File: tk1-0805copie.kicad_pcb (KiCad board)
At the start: 2 copper layers, 63 x 38.4 mm, 65 parts, among them P1 USB_C_Plug, U1 MCP1824T-2502EOT, U2 NCV8164ASN120T1G, U3 CH552E, U5 USBLC6-2SC6, U6 ICE40UP5K-SG48ITR, U8 W25Q80DVSNIG, U9 NCP752BSN33T1G

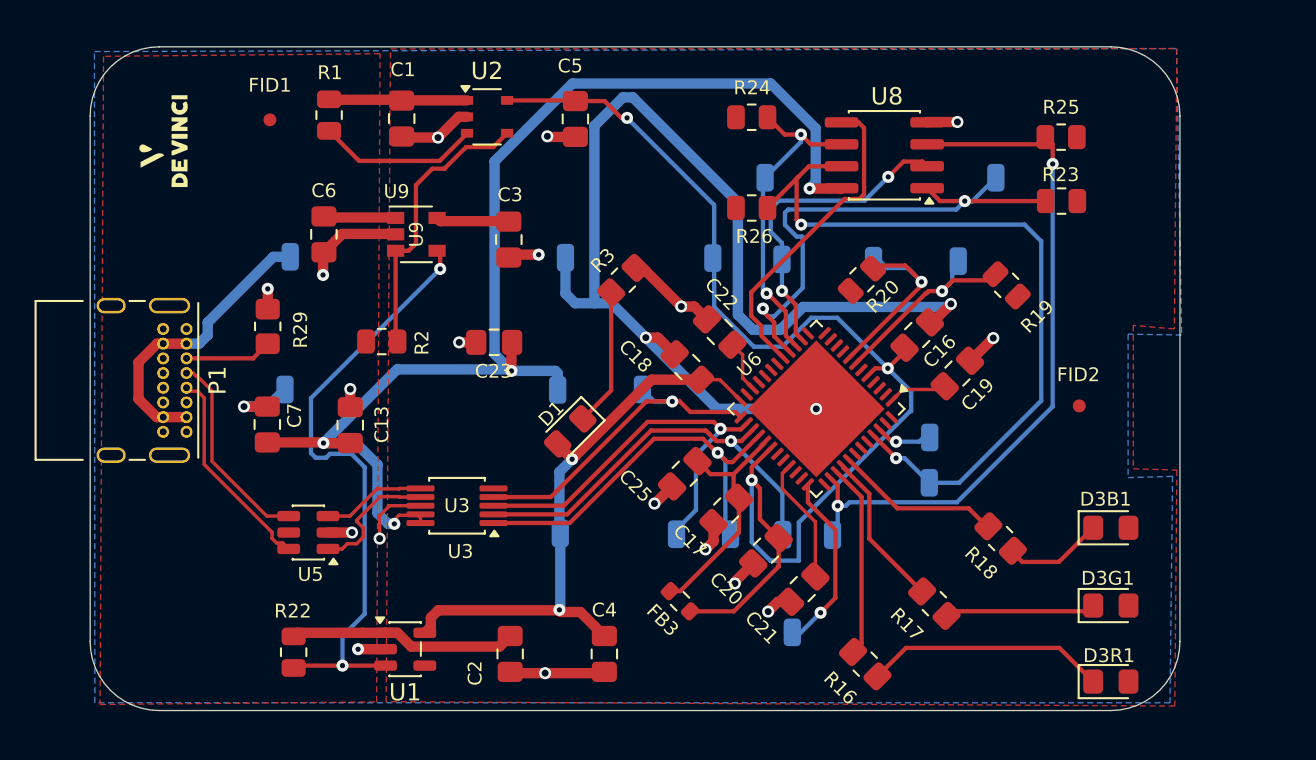
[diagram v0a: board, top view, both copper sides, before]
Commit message: Mise à jour du projet
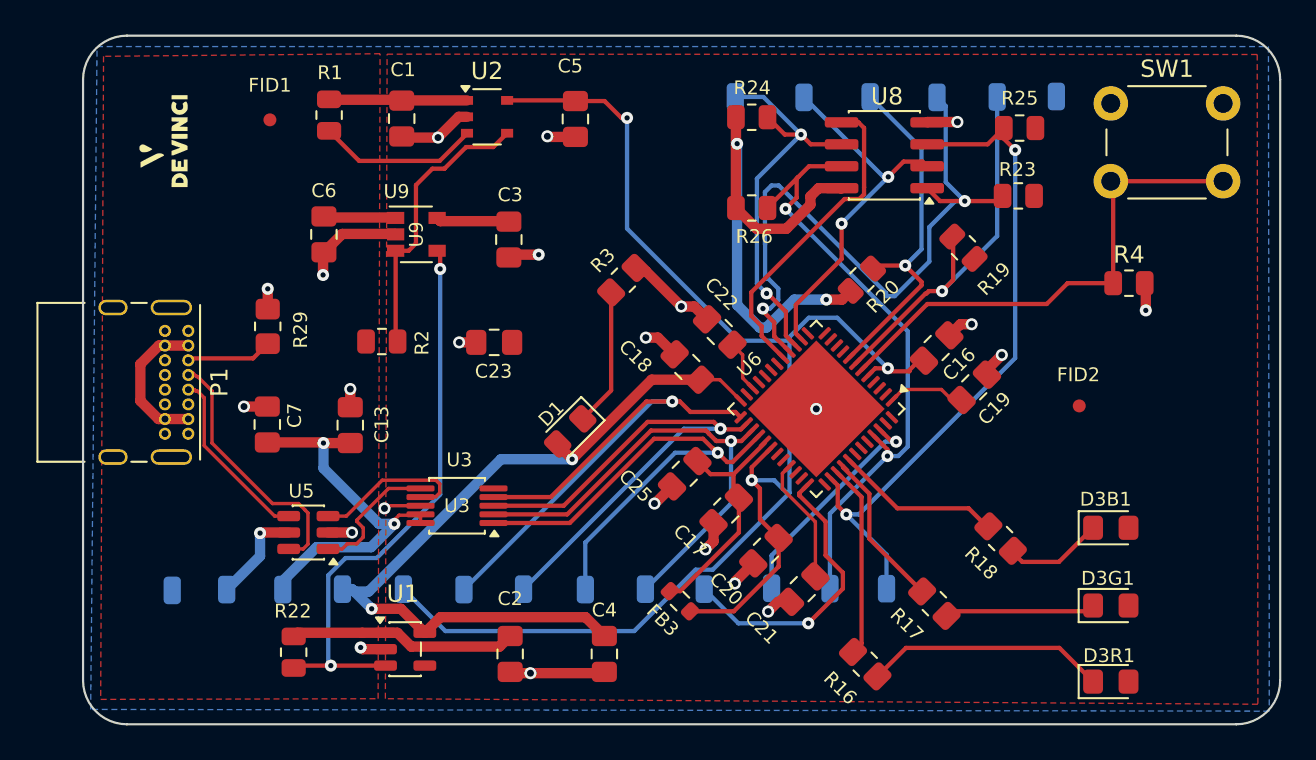
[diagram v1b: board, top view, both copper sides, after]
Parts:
- added R4: 10k, Resistor_SMD:R_0805_2012Metric, F.Cu at (138.1, 86.8)
- added SW1: SW_Push, Button_Switch_THT:SW_PUSH_6mm, F.Cu at (137.0, 76.3)
- U8: value W25Q80DVSNIG -> SST26VF080A-104I/SN
- moved TP5 29.9 mm to (133.8, 76.0)
- moved TP4 26.2 mm to (96.1, 104.5)
- moved TP2 19.7 mm to (89.1, 104.5)
- moved TP1 19.6 mm to (85.8, 104.5)
- moved TP6 15.5 mm to (99.6, 104.5)
- moved TP28 13.3 mm to (82.7, 104.5)
- moved TP3 13.0 mm to (92.5, 104.5)
- moved TP21 12.6 mm to (117.4, 104.4)
- moved TP17 9.76 mm to (130.4, 76.0)
- moved TP16 9.48 mm to (123.1, 76.0)
- moved TP15 9.46 mm to (119.2, 76.0)
- moved TP7 9.40 mm to (103.0, 104.5)
- moved TP8 8.99 mm to (106.6, 104.5)
- moved TP9 8.55 mm to (110.1, 104.5)
- moved TP20 8.40 mm to (120.8, 104.4)
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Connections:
- U3 pad 6: INT_USB_D- -> INT_USB_D+
- U3 pad 7: INT_USB_D+ -> INT_USB_D-
- U5 pad 4: /USB to Serial converter/INT_USB_IN_D+ -> /USB to Serial converter/INT_USB_IN_D-
- U5 pad 6: /USB to Serial converter/INT_USB_IN_D- -> /USB to Serial converter/INT_USB_IN_D+
- U6 pad : (no net) -> APP_GPIO1
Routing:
- net GND: track 113.4 -> 48.9 mm, vias 22 -> 23
- net TOUCH_EVENT: track 0.00 -> 29.1 mm
- net +3.3V: track 90.3 -> 72.0 mm
- net +1V2: track 71.7 -> 89.3 mm
- net INTERFACE_TX: track 19.0 -> 33.5 mm
- net +2V5: track 34.3 -> 46.2 mm
- net APP_CDONE: track 12.4 -> 22.8 mm
- net APP_GPIO4: track 3.29 -> 13.1 mm
- net APP_ICE_SS: track 31.6 -> 40.3 mm
- net /Application FPGA/APP_FLASH_HOLD: track 44.7 -> 36.3 mm
- net APP_CRESET: track 12.7 -> 20.8 mm
- net INTERFACE_RX: track 24.1 -> 32.2 mm
- net INTERFACE_RTS: track 23.8 -> 31.4 mm
- net APP_GPIO1: track 10.7 -> 17.1 mm
- net APP_ICE_SCK: track 18.9 -> 23.9 mm
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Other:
- board size 63 x 38.4 mm -> 69.3 x 39.8 mm
